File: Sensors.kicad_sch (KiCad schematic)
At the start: 32 parts, among them J16 SM02B-GHS-TB, J17 SM02B-GHS-TB, J18 SM02B-GHS-TB, J19 SM02B-GHS-TB, Q2 2N7002, U13 BME280, U16 BNO085, U19 BME280, U7 BNO085

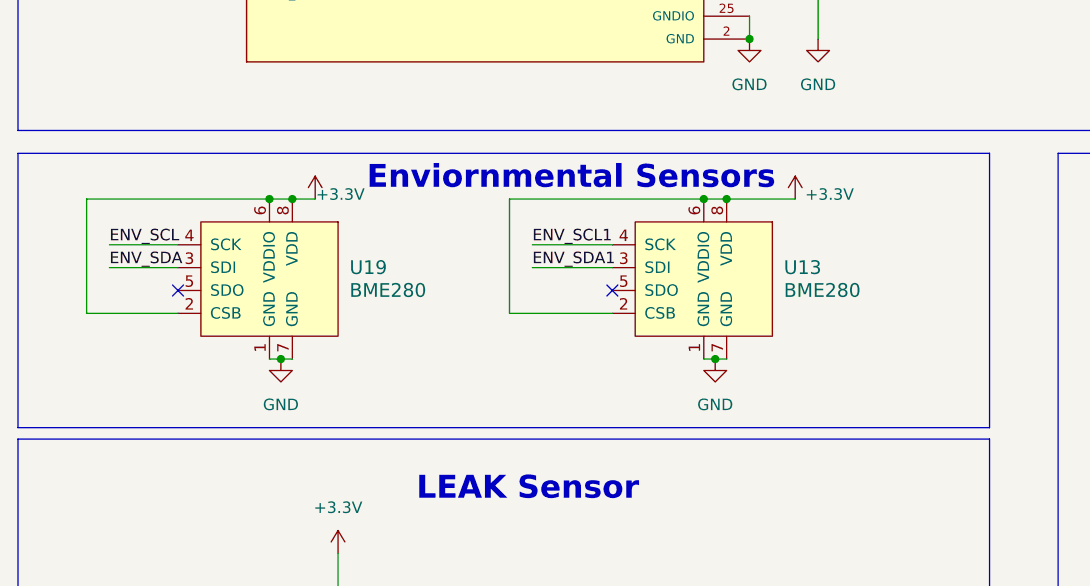
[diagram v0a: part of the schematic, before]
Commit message: stuff
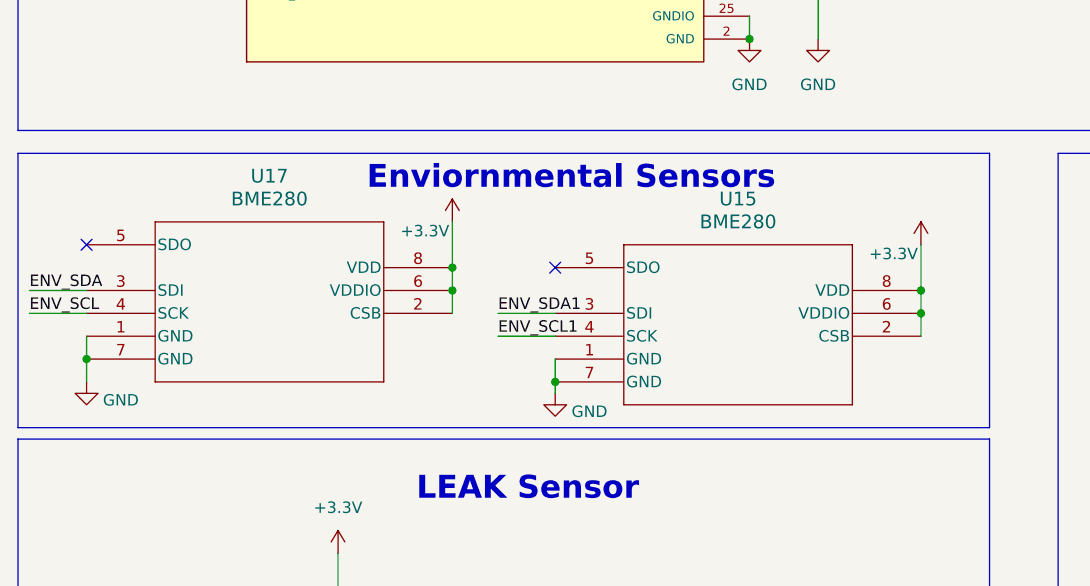
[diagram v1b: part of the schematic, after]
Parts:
- removed U13, U19: BME280, digikey-footprints:Pressure_Sensor_LGA-8_2.5x2.5mm_BME280, symbol dk_Humidity-Moisture-Sensors:BME280
- added U15, U17: BME280, BME280:DFN8_0p65_2p5SQ_BOS, symbol BME280:BME280
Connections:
- net +3.3V: now also U15.2 (CSB), U15.6 (VDDIO), U15.8 (VDD), U17.2 (CSB), U17.6 (VDDIO), U17.8 (VDD)
- net ENV_SCL: now also U17.4 (SCK)
- net ENV_SCL1: now also U15.4 (SCK)
- net ENV_SDA: now also U17.3 (SDI)
- net ENV_SDA1: now also U15.3 (SDI)
- net GND: now also U15.1 (GND), U15.7 (GND), U17.1 (GND), U17.7 (GND)
